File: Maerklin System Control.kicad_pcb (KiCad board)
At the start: 2 copper layers, 83.8 x 73 mm, 33 parts, among them J1 Female Header, J2 Input, J3 Output, J4 Conn_S3 Mini, SW1 UP, SW2 RIGHT, SW3 DOWN, SW4 LEFT, SW5 SELECT, SW6 BACK

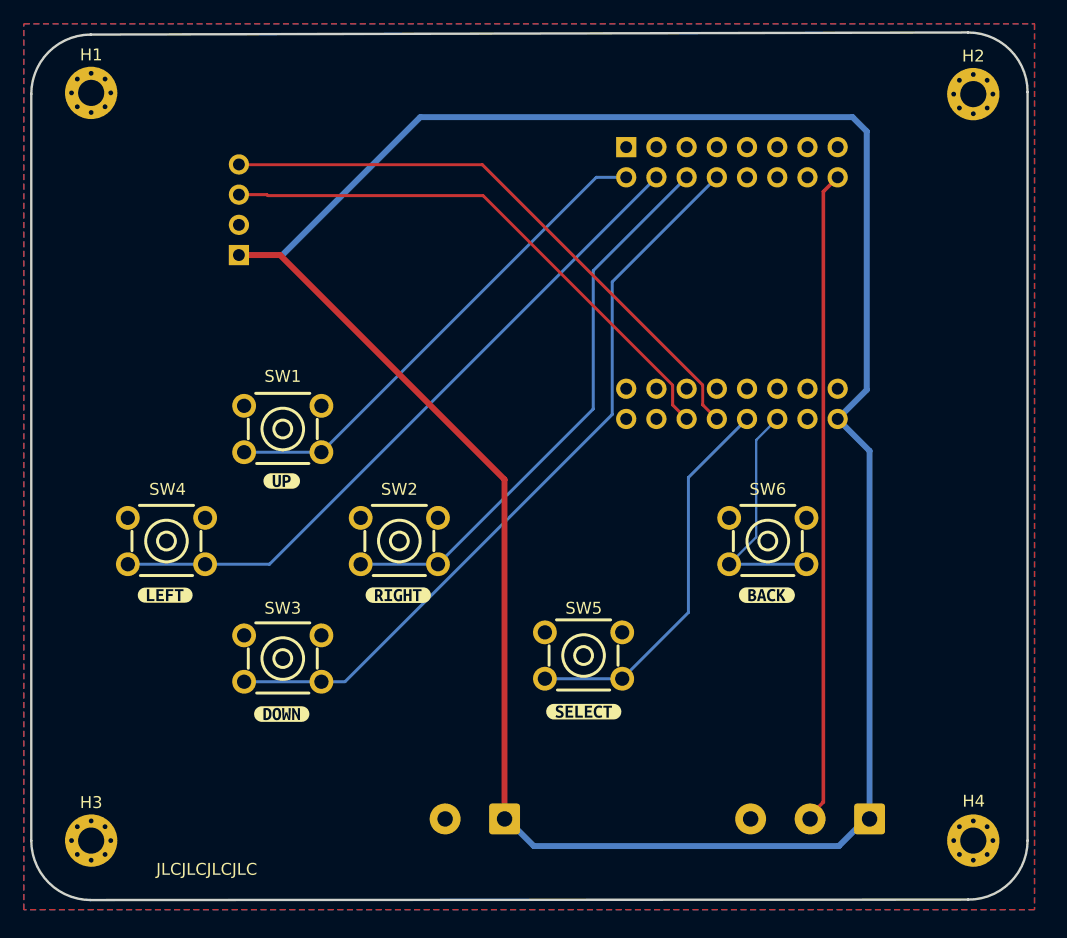
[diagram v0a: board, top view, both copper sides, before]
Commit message: RC of mk2
Signed-off-by: Peter Siegmund <mars3142@users.noreply.github.com>
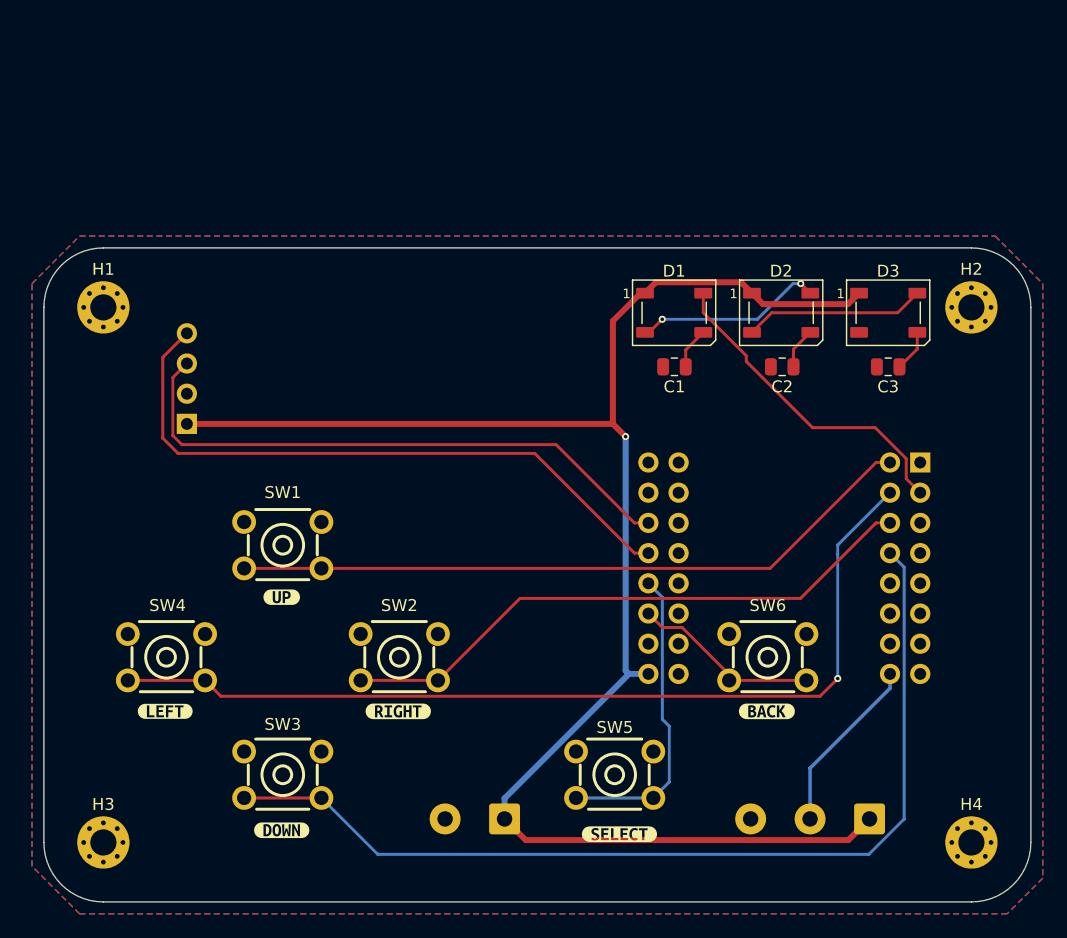
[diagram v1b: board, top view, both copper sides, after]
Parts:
- removed kibuzzard-67E5658B: G***, kibuzzard-67E5658B
- added C1: 100nF, Capacitor_SMD:C_0805_2012Metric, F.Cu at (115.6, 50.8)
- added C2: 100nF, Capacitor_SMD:C_0805_2012Metric, F.Cu at (124.7, 50.9)
- added C3: 100nF, Capacitor_SMD:C_0805_2012Metric, F.Cu at (133.6, 50.9)
- added D1: WS2812B, LED_SMD:LED_WS2812B_PLCC4_5.0x5.0mm_P3.2mm, F.Cu at (115.6, 46.3)
- added D2: WS2812B, LED_SMD:LED_WS2812B_PLCC4_5.0x5.0mm_P3.2mm, F.Cu at (124.6, 46.3)
- added D3: WS2812B, LED_SMD:LED_WS2812B_PLCC4_5.0x5.0mm_P3.2mm, F.Cu at (133.6, 46.3)
- added kibuzzard-6859B258: G***, kibuzzard-6859B258, B.Cu at (77.3, 51.9)
- moved kibuzzard-67897FC0 26.0 mm to (129.6, 67.7), turned to 90 degrees
- moved J4 24.1 mm to (124.6, 67.9), turned to 180 degrees
- moved H1 18.1 mm to (67.6, 45.9)
- moved H2 17.9 mm to (140.6, 45.9)
- moved kibuzzard-67898074 14.9 mm to (71.2, 53.1)
- moved kibuzzard-67898084 14.9 mm to (71.2, 55.7)
- moved kibuzzard-67898040 14.9 mm to (71.2, 47.9)
- moved kibuzzard-67898062 14.9 mm to (71.2, 50.5)
- moved J1 14.9 mm to (74.6, 55.7)
- moved kibuzzard-678981DB 10.7 mm to (111.0, 90.2)
- moved SW5 10.4 mm to (110.6, 85.2)
- moved kibuzzard-678981FB 9.77 mm to (123.4, 79.8)
- moved kibuzzard-67898208 9.77 mm to (82.6, 70.2)
- moved kibuzzard-67898217 9.77 mm to (82.6, 89.8)
- moved kibuzzard-67898221 9.77 mm to (72.8, 79.8)
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- renumbered J3 to J2, J2 to J3
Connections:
- J4 pad 2: unconnected-(J4-IO2-Pad2) -> LED
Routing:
- net +5V: track 209.2 -> 139.6 mm, vias 0 -> 1
- net DOUT: track 54.7 -> 15.0 mm
- net LED: track 0.00 -> 27.4 mm
- net LEFT: track 57.9 -> 78.3 mm, vias 0 -> 1
- net DOWN: track 63.9 -> 81.6 mm
- net UP: track 41.7 -> 58.0 mm
- net Net-(D1-DOUT): track 0.00 -> 15.9 mm, vias 0 -> 2
- net Net-(D2-DOUT): track 0.00 -> 15.3 mm
- net SELECT: track 32.7 -> 25.8 mm
- net BACK: track 20.4 -> 15.9 mm
- net SDA: track 50.0 -> 54.5 mm
- net Net-(D3-VSS): track 0.00 -> 3.52 mm
- net Net-(D1-VSS): track 0.00 -> 3.51 mm
- net Net-(D2-VSS): track 0.00 -> 3.48 mm
- net SCK: track 46.4 -> 49.6 mm
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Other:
- board size 83.8 x 73 mm -> 83 x 55 mm
- board text added: "System Control MK2"
- board text removed: "JLCJLCJLCJLC"
- board text removed: "System Control MK1.1"
